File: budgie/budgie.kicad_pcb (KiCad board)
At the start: 2 copper layers, 126.8 x 80.5 mm, 15 parts

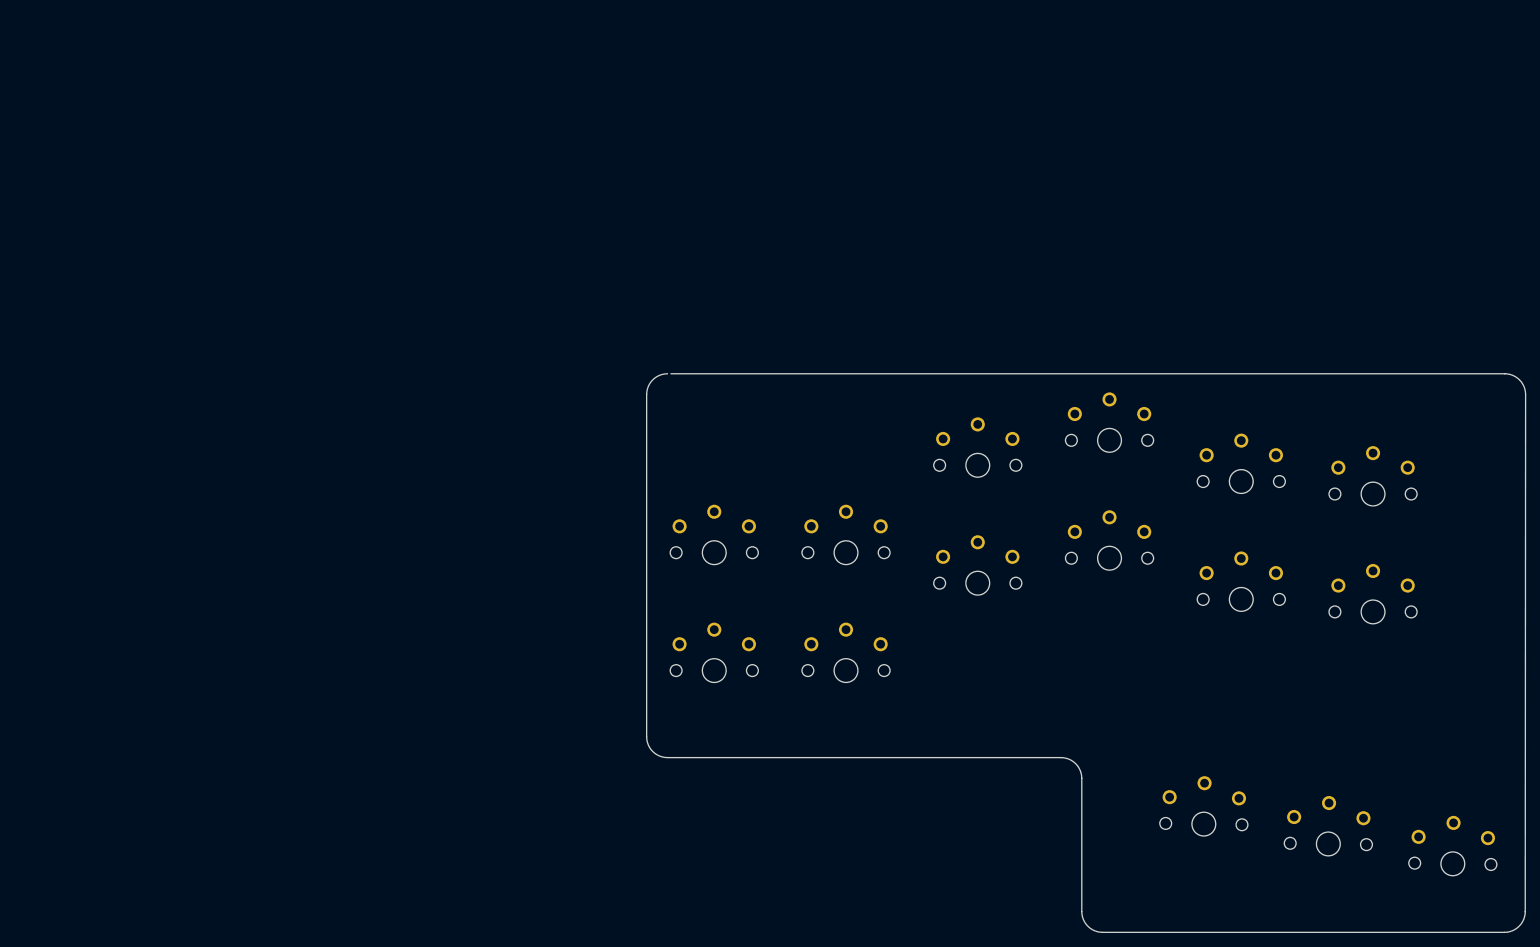
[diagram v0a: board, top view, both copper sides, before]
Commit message: updates
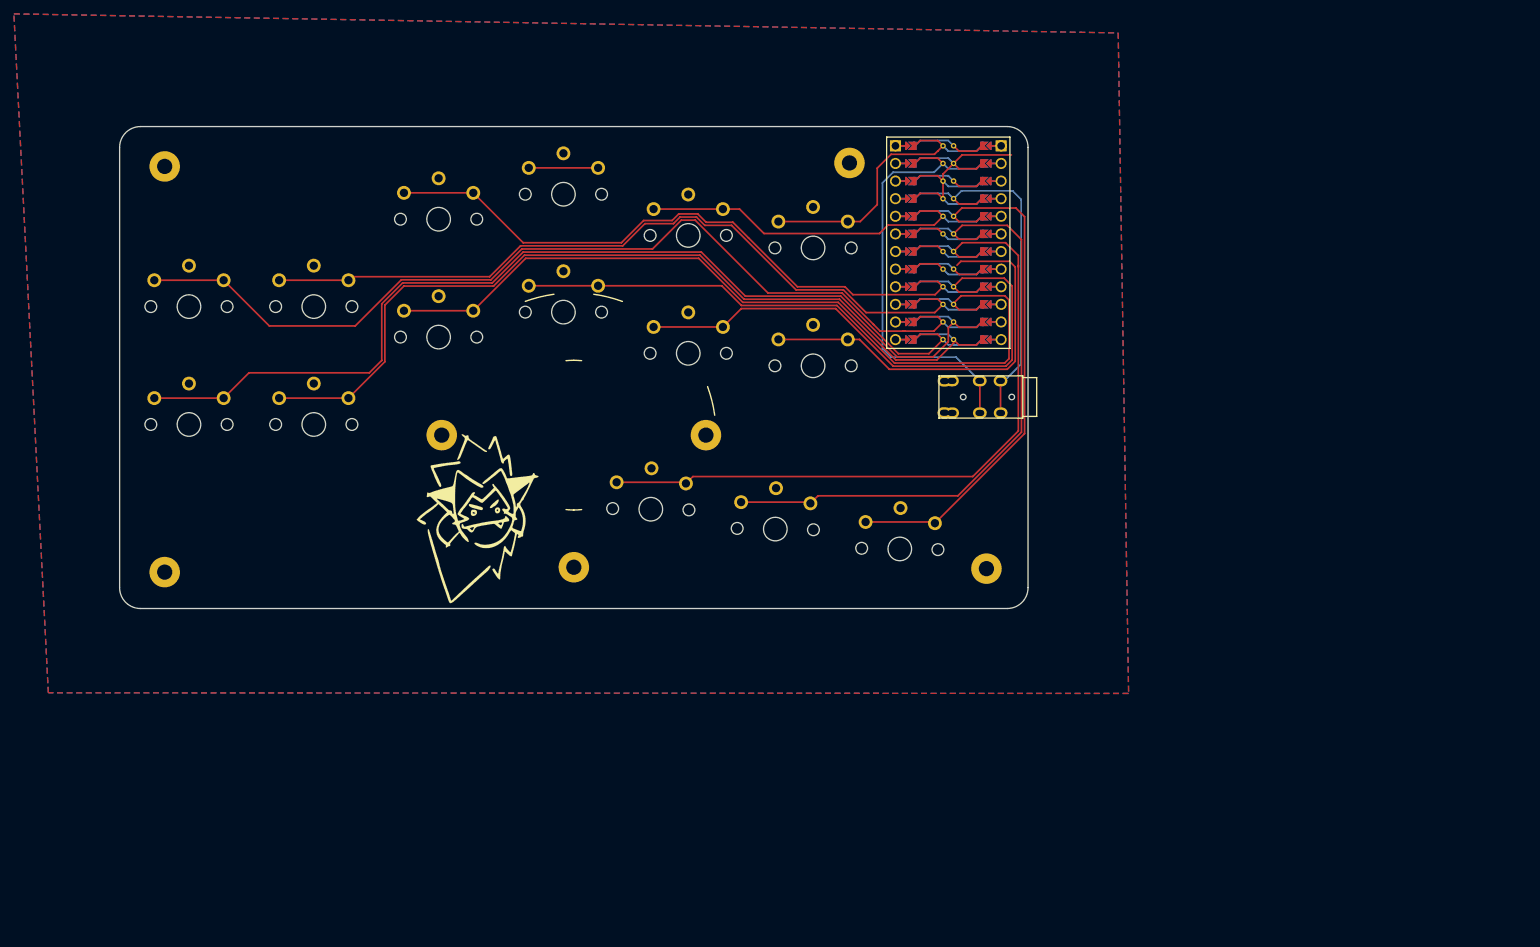
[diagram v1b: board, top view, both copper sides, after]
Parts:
- added ?: , , F.Cu at (173.0, 108.0)
- added ?: , , F.Cu at (153.2, 49.5)
- added ?: , , F.Cu at (54.5, 108.5)
- added ?: , , F.Cu at (54.5, 50.0)
- added J2: AudioJack4dpb, Kailh:TRRS-PJ-DPB2, F.Cu at (178.2, 83.2)
- added REF**: Tenting Puck, trochilidae:Tenting_Puck2, F.Cu at (113.5, 88.8)
- added Ref**: Val**, img:catra, F.Cu at (99.2, 100.8)
- added Ref**: Val**, img:adora, B.Cu at (99.7, 99.0)
- added U1: ProMicro-kbd, * duckyb-collection:ProMicro_jumpers_facedown, F.Cu at (167.5, 61.0)
- S1, S10, S11, S12, S13, S14, S15, S2, S3, S4, S5, S6, S7, S8, S9: footprint PG1350 -> pg1350:pg1350-R
- moved S13 91.8 mm to (124.6, 99.4)
- moved S14 91.8 mm to (142.6, 102.3)
- moved S15 91.8 mm to (160.5, 105.2)
- moved S11 88.2 mm to (148.0, 78.8)
- moved S12 88.2 mm to (148.0, 61.8)
- moved S10 87.3 mm to (130.0, 60.0)
- moved S9 87.3 mm to (130.0, 77.0)
- moved S7 86.4 mm to (112.0, 71.0)
- moved S8 86.4 mm to (112.0, 54.0)
- moved S5 85.5 mm to (94.0, 74.6)
- moved S6 85.5 mm to (94.0, 57.6)
- moved S3 84.6 mm to (76.0, 87.2)
- moved S4 84.6 mm to (76.0, 70.2)
- moved S1 83.7 mm to (58.0, 87.2)
- moved S2 83.7 mm to (58.0, 70.2)
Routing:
- net matrix_outer_bottom: track 0.00 -> 134.2 mm
- net matrix_outer_home: track 0.00 -> 130.2 mm
- net matrix_pinky_bottom: track 0.00 -> 119.9 mm
- net matrix_pinky_home: track 0.00 -> 105.7 mm
- net thumb_tucky: track 0.00 -> 97.3 mm
- net matrix_middle_bottom: track 0.00 -> 91.4 mm
- net matrix_ring_bottom: track 0.00 -> 90.0 mm
- net matrix_ring_home: track 0.00 -> 87.7 mm
- net thumb_homey: track 0.00 -> 83.7 mm
- net matrix_index_bottom: track 0.00 -> 76.7 mm
- net thumb_reachy: track 0.00 -> 70.9 mm
- net matrix_inner_bottom: track 0.00 -> 59.0 mm
- net RX: track 0.00 -> 54.4 mm
- net matrix_index_home: track 0.00 -> 44.2 mm
- net VCC: track 0.00 -> 43.1 mm
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- added copper zone on B.Cu, net GND
- added copper zone on F.Cu, net GND
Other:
- board size 126.8 x 80.5 mm -> 131 x 69.5 mm
- rule pad_to_mask_clearance: 0.05 -> 0
